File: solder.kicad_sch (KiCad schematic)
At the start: 5 parts

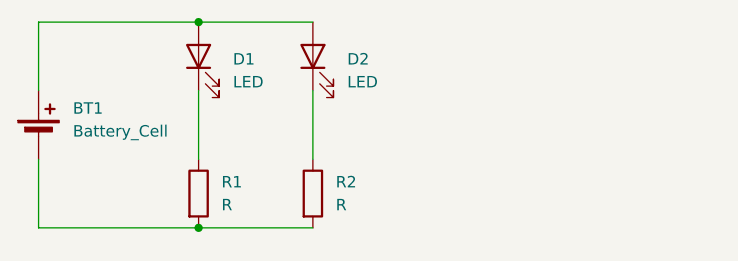
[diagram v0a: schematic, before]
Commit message: update!!! made LEDs blink
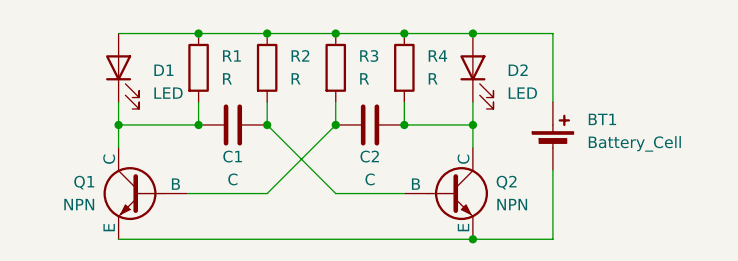
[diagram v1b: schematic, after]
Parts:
- added C1, C2: C, Capacitor_THT:CP_Radial_D8.0mm_P5.00mm, symbol Device:C
- added Q1, Q2: NPN, Package_TO_SOT_THT:TO-92L_HandSolder, symbol Simulation_SPICE:NPN
- added R3, R4: R, Resistor_THT:R_Axial_DIN0207_L6.3mm_D2.5mm_P7.62mm_Horizontal, symbol Device:R
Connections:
- net at R1.1: now also BT1.1 (+), D1.2 (A), D2.2 (A), R2.1, R3.1, R4.1; no longer D1.1 (K)
- net at D2.1 (K): now also C2.2, Q2.1 (C), R4.2; no longer R2.1
- new net: C2.1, Q1.2 (B), R3.2
- new net: C1.1, D1.1 (K), Q1.1 (C), R1.2
- new net: BT1.2 (-), Q1.3 (E), Q2.3 (E)
- new net: C1.2, Q2.2 (B), R2.2
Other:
- moved on the sheet: BT1, D1, D2, R1, R2
